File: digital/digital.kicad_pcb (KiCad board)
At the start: 2 copper layers, 52 x 68 mm, 128 parts, among them J101 BASEBAND, J102 LNA_INTERFACE, J103 VCO_INTERFACE, J104 RF_POWER, J105 UART, J106 PLL_INTERFACE, J107 PA_INTERFACE, J108 USB_OTG, J109 FPGA_PROG, J110 SWD/JTAG, J111 PWR_IN, Q101 Q_PMOS_GSD, U101 LDK320AM33R, U102 TPS54308, U201 STM32F070C6T6, U202 SG5032CAN8.000000M-TJGA3, U301 ICE5LP1K-SG48ITR50, U302 LFSPXO025559Reel, U303 AT25SF041, U304 TLV74125PDBVR, U305 TLV74312PDBVR, U401 ADS7057, U402 LDK320AM33R, U403 OPA2376QDGKRQ1

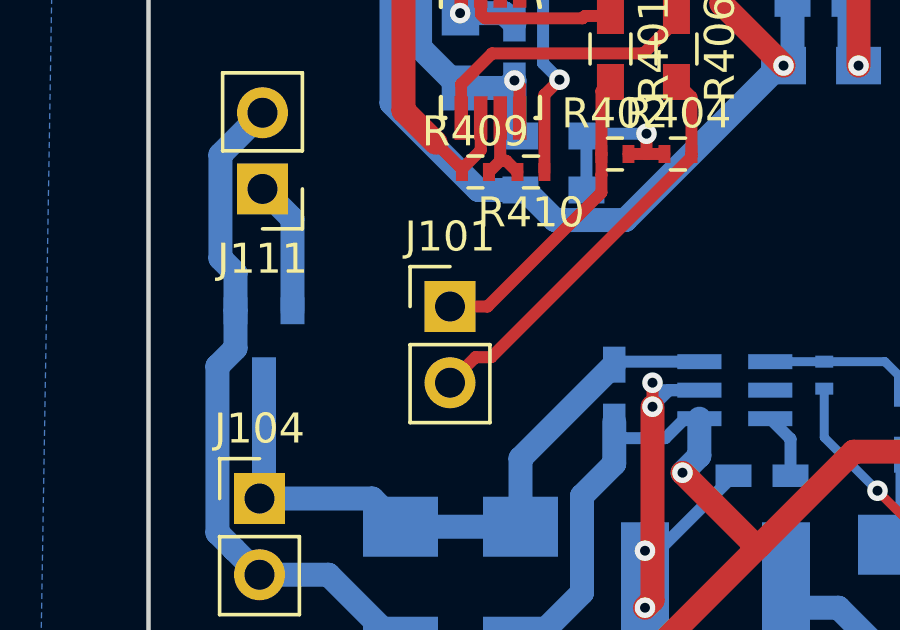
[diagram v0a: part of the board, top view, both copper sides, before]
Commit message: Regenerate Gerbers
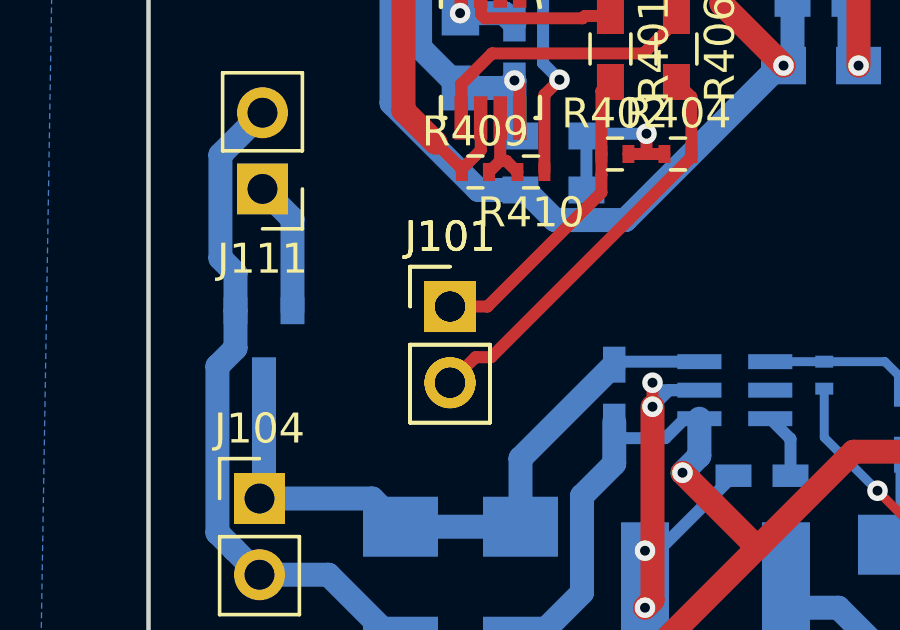
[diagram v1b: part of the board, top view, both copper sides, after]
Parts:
- added J101: BASEBAND, Pin_Headers:Pin_Header_Straight_1x02_Pitch2.54mm, F.Cu at (110.0, 153.5)
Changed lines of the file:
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@@
     (links 284)
     (no_connects 0)
-    (area 91.5 95.25 156.950001 174.900001)
+    (area 99.924999 99.924999 152.075001 168.075001)
     (thickness 1.6)
     (drawings 4)
     (tracks 1202)
     (zones 0)
-    (modules 128)
+    (modules 129)
     (nets 71)
   )
@@
   )
   (setup
-    (last_trace_width 0.8)
+    (last_trace_width 0.1524)
     (user_trace_width 0.3)
     (user_trace_width 0.4)
@@
     (visible_elements FFFFFF7F)
     (pcbplotparams
-      (layerselection 0x00030_80000001)
+      (layerselection 0x01030_80000001)
       (usegerberextensions false)
       (excludeedgelayer true)
@@
       (outputformat 1)
       (mirror false)
-      (drillshape 1)
+      (drillshape 0)
       (scaleselection 1)
-      (outputdirectory ""))
+      (outputdirectory ../gerber/))
   )
   (net 0 "")
@@
     (add_net VBUS)
   )
+  (module Pin_Headers:Pin_Header_Straight_1x02_Pitch2.54mm (layer F.Cu)
+    (at 110.05 153.46)
+    (descr "Through hole straight pin header, 1x02, 2.54mm pitch, single row")
+    (tags "Through hole pin header THT 1x02 2.54mm single row")
+    (fp_text reference J101 (at 0 -2.33) (layer F.SilkS)
+      (effects (font (size 1 1) (thickness 0.15)))
+    )
+    (fp_text value BASEBAND (at 0 4.87) (layer F.Fab)
+      (effects (font (size 1 1) (thickness 0.15)))
+    )
+    (fp_line (start -0.635 -1.27) (end 1.27 -1.27) (layer F.Fab) (width 0.1))
+    (fp_line (start 1.27 -1.27) (end 1.27 3.81) (layer F.Fab) (width 0.1))
+    (fp_line (start 1.27 3.81) (end -1.27 3.81) (layer F.Fab) (width 0.1))
+    (fp_line (start -1.27 3.81) (end -1.27 -0.635) (layer F.Fab) (width 0.1))
+    (fp_line (start -1.27 -0.635) (end -0.635 -1.27) (layer F.Fab) (width 0.1))
+    (fp_line (start -1.33 3.87) (end 1.33 3.87) (layer F.SilkS) (width 0.12))
+    (fp_line (start -1.33 1.27) (end -1.33 3.87) (layer F.SilkS) (width 0.12))
+    (fp_line (start 1.33 1.27) (end 1.33 3.87) (layer F.SilkS) (width 0.12))
+    (fp_line (start -1.33 1.27) (end 1.33 1.27) (layer F.SilkS) (width 0.12))
+    (fp_line (start -1.33 0) (end -1.33 -1.33) (layer F.SilkS) (width 0.12))
+    (fp_line (start -1.33 -1.33) (end 0 -1.33) (layer F.SilkS) (width 0.12))
+    (fp_line (start -1.8 -1.8) (end -1.8 4.35) (layer F.CrtYd) (width 0.05))
+    (fp_line (start -1.8 4.35) (end 1.8 4.35) (layer F.CrtYd) (width 0.05))
+    (fp_line (start 1.8 4.35) (end 1.8 -1.8) (layer F.CrtYd) (width 0.05))
+    (fp_line (start 1.8 -1.8) (end -1.8 -1.8) (layer F.CrtYd) (width 0.05))
+    (fp_text user %R (at 0 1.27 90) (layer F.Fab)
+      (effects (font (size 1 1) (thickness 0.15)))
+    )
+    (pad 1 thru_hole rect (at 0 0) (size 1.7 1.7) (drill 1) (layers *.Cu *.Mask)
+      (net 28 /ADC/IN+))
+    (pad 2 thru_hole oval (at 0 2.54) (size 1.7 1.7) (drill 1) (layers *.Cu *.Mask)
+      (net 29 /ADC/IN-))
+    (model ${KISYS3DMOD}/Pin_Headers.3dshapes/Pin_Header_Straight_1x02_Pitch2.54mm.wrl
+      (at (xyz 0 0 0))
+      (scale (xyz 1 1 1))
+      (rotate (xyz 0 0 0))
+    )
+  )
   (module Capacitors_SMD:C_0805_HandSoldering (layer B.Cu)
